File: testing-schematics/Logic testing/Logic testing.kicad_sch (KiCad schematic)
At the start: 19 parts, among them J1 Fencer's Wire, J2 Opponent's Wire, J3 Wire Test, J4 Lame Tab, K1 G6K-2, K2 G6K-2, K3 G6K-2, Q1 BC547, Q2 BC547, Q3 BC547

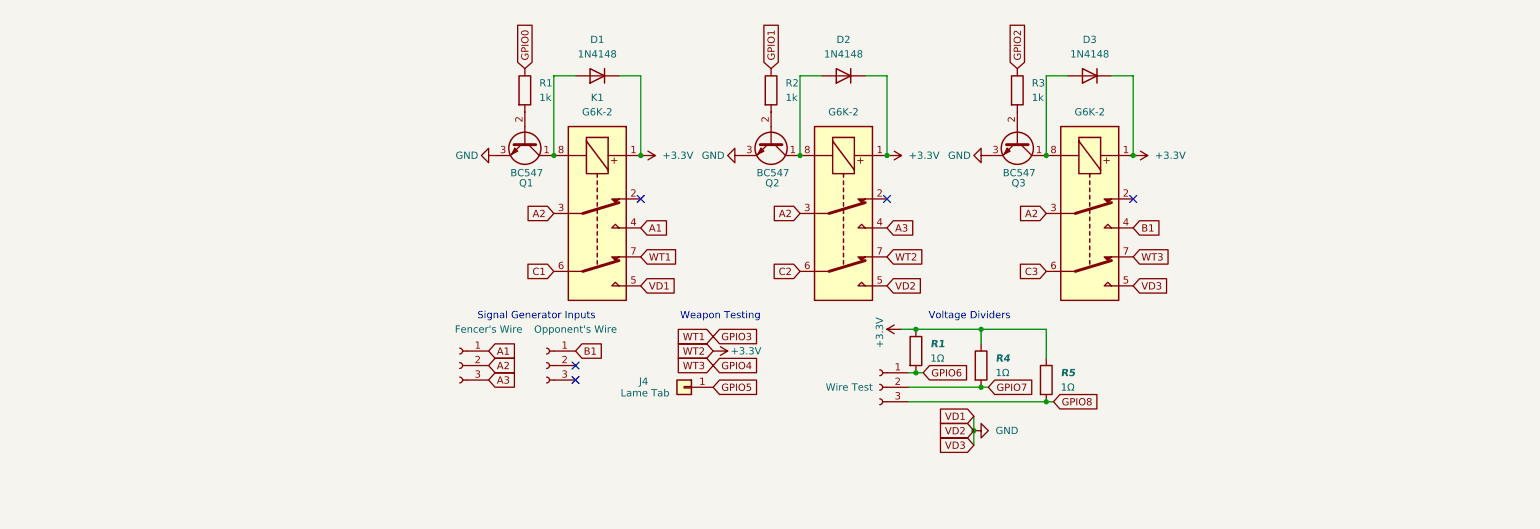
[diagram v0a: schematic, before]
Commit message: Update schematic and BOM
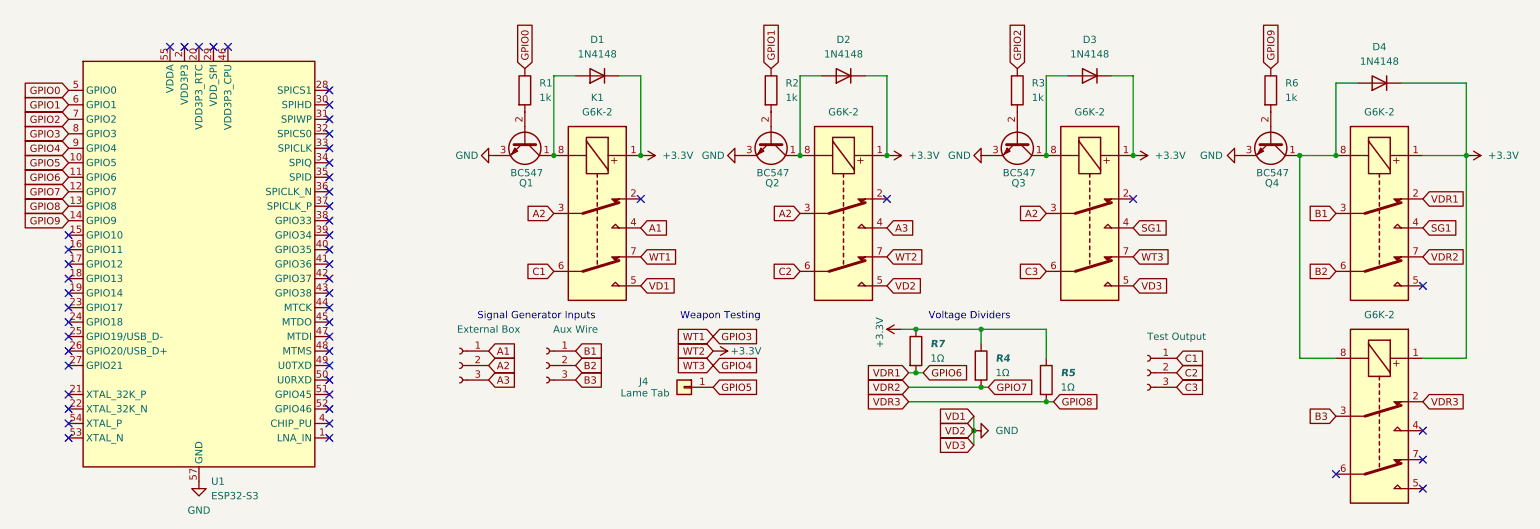
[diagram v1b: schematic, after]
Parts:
- removed J3: Wire Test, symbol Connector:Conn_01x03_Socket
- added D4: 1N4148, Diode_THT:D_DO-35_SOD27_P7.62mm_Horizontal, symbol Diode:1N4148
- added J5: Test Output, symbol Connector:Conn_01x03_Socket
- added K4, K5: G6K-2, symbol Relay:G6K-2
- added Q4: BC547, Package_TO_SOT_THT:TO-92_Inline, symbol Transistor_BJT:BC547
- added R6: 1k, Resistor_THT:R_Axial_DIN0204_L3.6mm_D1.6mm_P7.62mm_Horizontal, symbol Device:R
- added U1: ESP32-S3, Package_DFN_QFN:QFN-56-1EP_7x7mm_P0.4mm_EP4x4mm, symbol MCU_Espressif:ESP32-S3
- J1: value Fencer's Wire -> External Box
- J2: value Opponent's Wire -> Aux Wire
- J4: footprint (none) -> Connector_Wire:SolderWire-0.5sqmm_1x01_D0.9mm_OD2.1mm
- R1, R2, R3, R4, R5: footprint (none) -> Resistor_THT:R_Axial_DIN0204_L3.6mm_D1.6mm_P7.62mm_Horizontal
- R7: renamed from R1; footprint (none) -> Resistor_THT:R_Axial_DIN0204_L3.6mm_D1.6mm_P7.62mm_Horizontal
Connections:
- net +3.3V: now also D4.1 (K), K4.1, K5.1
- net B1: now also K4.3; no longer K3.4
- net C1: now also J5.1 (Pin_1)
- net C2: now also J5.2 (Pin_2)
- net C3: now also J5.3 (Pin_3)
- net GND: now also Q4.3 (E), U1.57 (GND)
- net GPIO0: now also U1.5 (GPIO0)
- net GPIO1: now also U1.6 (GPIO1)
- net GPIO2: now also U1.7 (GPIO2)
- net GPIO3: now also U1.8 (GPIO3)
- net GPIO4: now also U1.9 (GPIO4)
- net GPIO5: now also U1.10 (GPIO5)
- net GPIO6: now also K4.2, U1.11 (GPIO6)
- net GPIO7: now also K4.7, U1.12 (GPIO7)
- net GPIO8: now also K5.2, U1.13 (GPIO8)
- net B2: now reaches J2.2 (Pin_2)
- net B2: now also K4.6
- net B3: now reaches J2.3 (Pin_3)
- net B3: now also K5.3
- new net: D4.2 (A), K4.8, K5.8, Q4.1 (C)
- new net: Q4.2 (B), R6.2
- new net: U1.2 (VDD3P3), U1.3 (VDD3P3)
- new net: U1.55 (VDDA), U1.56 (VDDA)
- new net GPIO9: R6.1, U1.14 (GPIO9)
- new net SG1: K3.4, K4.4
- no-connect marks 5 -> 52
